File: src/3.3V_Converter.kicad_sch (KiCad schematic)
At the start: 16 parts, among them U4 TPS566238RQFR

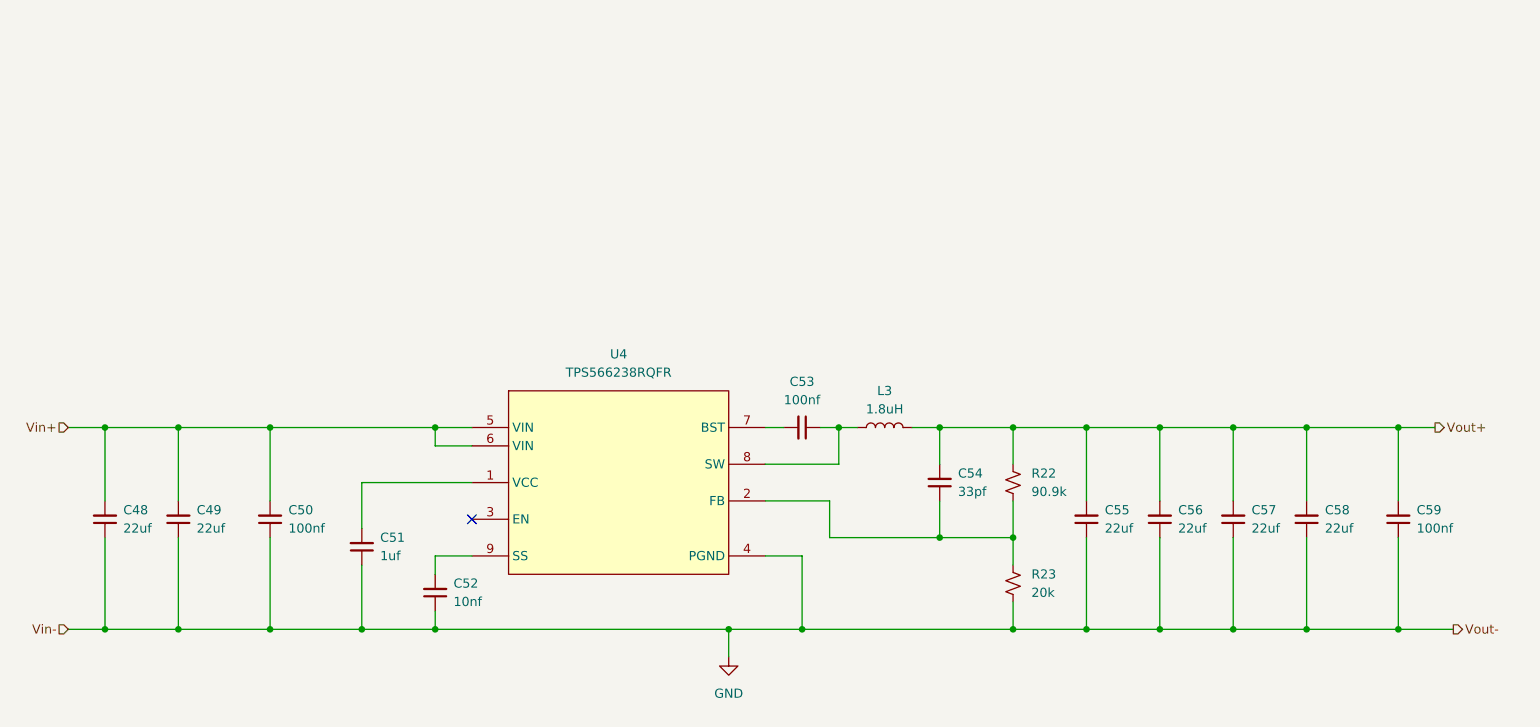
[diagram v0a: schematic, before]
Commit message: GG
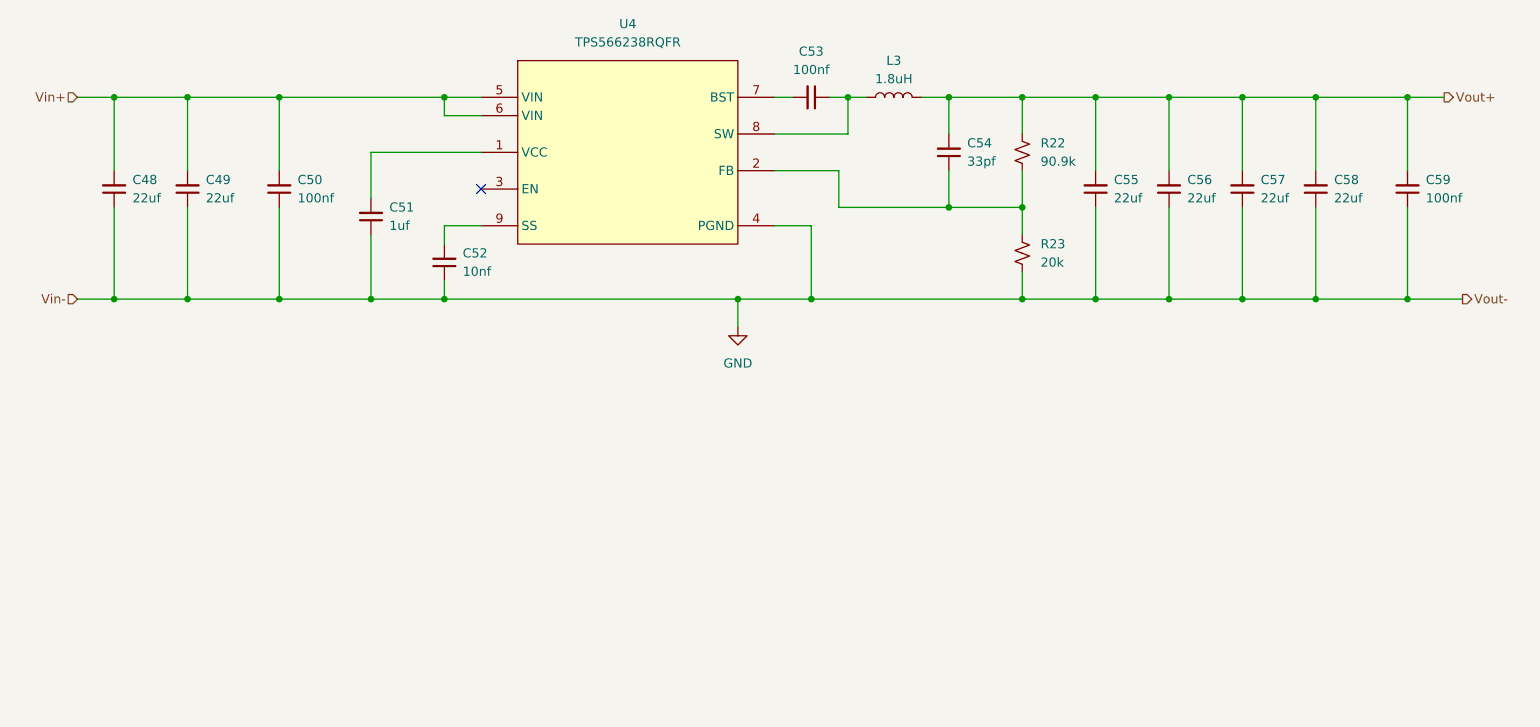
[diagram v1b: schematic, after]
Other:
- moved on the sheet: C48, C49, C50, C51, C52, C53, C54, C55, C56, C57, C58, C59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

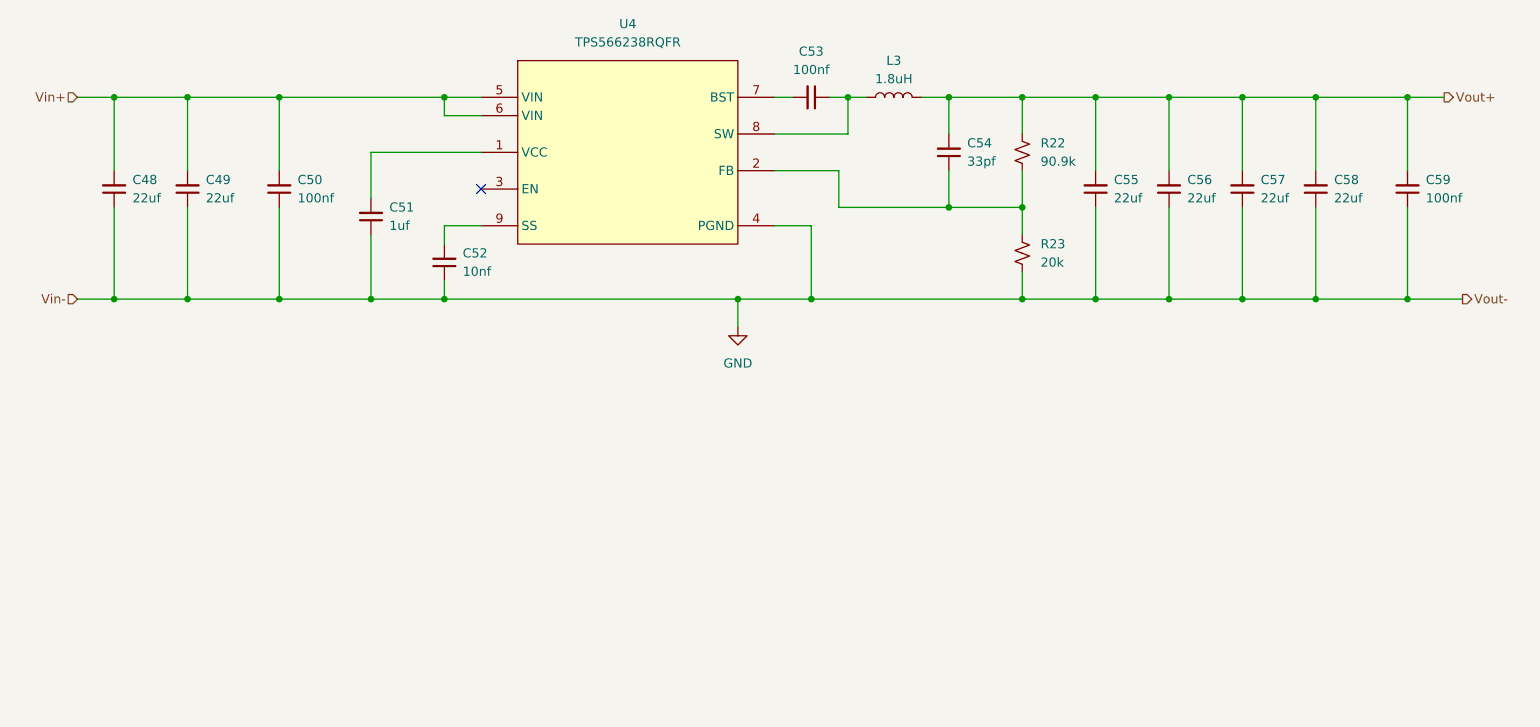
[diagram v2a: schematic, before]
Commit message: Completed half of the PCB layout
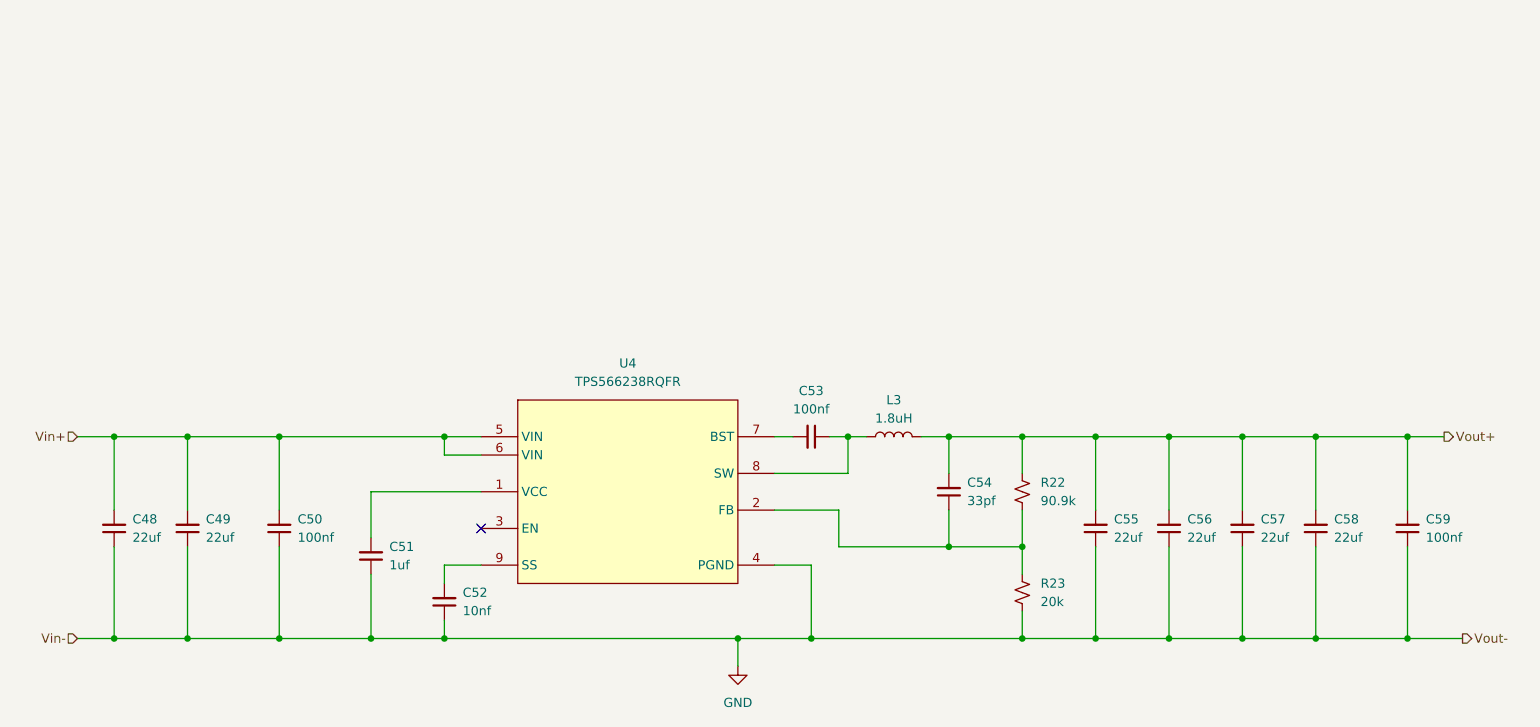
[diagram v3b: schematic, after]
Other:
- moved on the sheet: C48, C49, C50, C51, C52, C53, C54, C55, C56, C57, C58, C59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

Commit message: Upated parts and BOM
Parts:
- C48, C49, C55, C56, C57, C58: LCSC Part (none) -> C5677683; MPN (none) -> MSAST21GBB5226MTNC12; Manufacturer (none) -> Taiyo Yuden
- C50, C59: LCSC Part (none) -> C108079; MPN (none) -> CC0603KRX7R7BB104; Manufacturer (none) -> YAGEO
- C51: LCSC Part (none) -> C2180996; MPN (none) -> C0603C105Z8VACTU; Manufacturer (none) -> KEMET
- C52: LCSC Part (none) -> C85735; MPN (none) -> GRM155R71C103KA01D; Manufacturer (none) -> Murata Electronics
- C53: LCSC Part (none) -> C71629; MPN (none) -> GRM155R71C104KA88D; Manufacturer (none) -> Murata Electronics
- C54: footprint Capacitor_SMD:C_0603_1608Metric -> Capacitor_SMD:C_0201_0603Metric; LCSC Part (none) -> C513616; MPN (none) -> CC0201JRNPO8BN330; Manufacturer (none) -> YAGEO
- L3: LCSC Part (none) -> C3911679; MPN (none) -> XAL7070-182MEC; Manufacturer (none) -> Coilcraft
- R22: LCSC Part (none) -> C2078245; MPN (none) -> ERJ6ENF9092V; Manufacturer (none) -> PANASONIC
- R23: LCSC Part (none) -> C844940; MPN (none) -> CRCW080520K0FKEA; Manufacturer (none) -> Vishay Intertech
- U4: LCSC Part (none) -> C5219353; MPN (none) -> TPS566238RQFR; Manufacturer (none) -> Texas Instruments
